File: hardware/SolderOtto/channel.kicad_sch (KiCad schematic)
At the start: 16 parts, among them J601 Conn_01x07

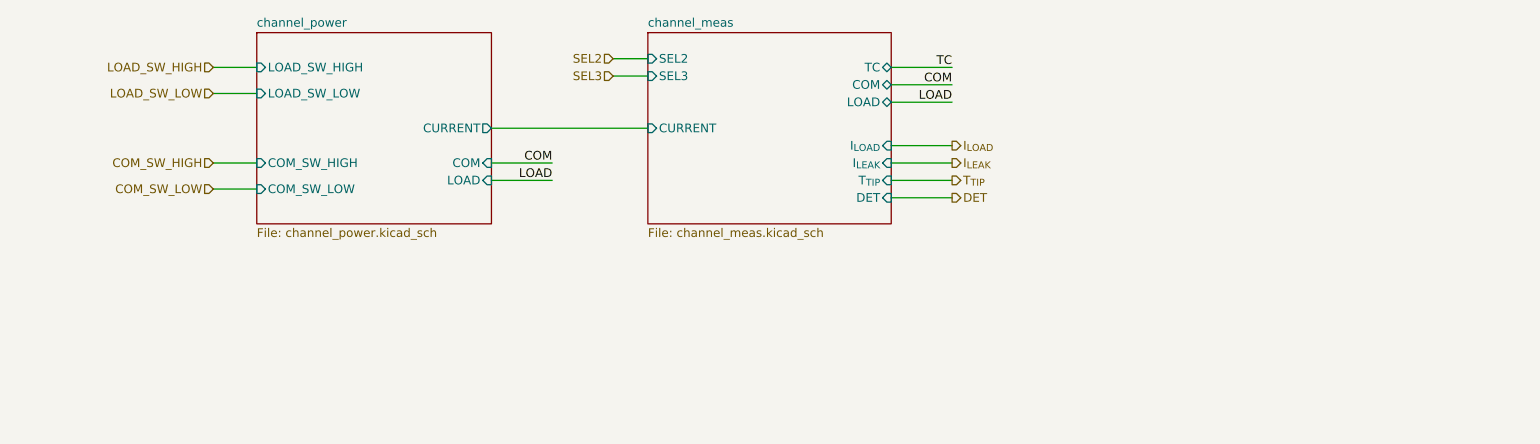
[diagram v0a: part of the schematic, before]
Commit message: save wip
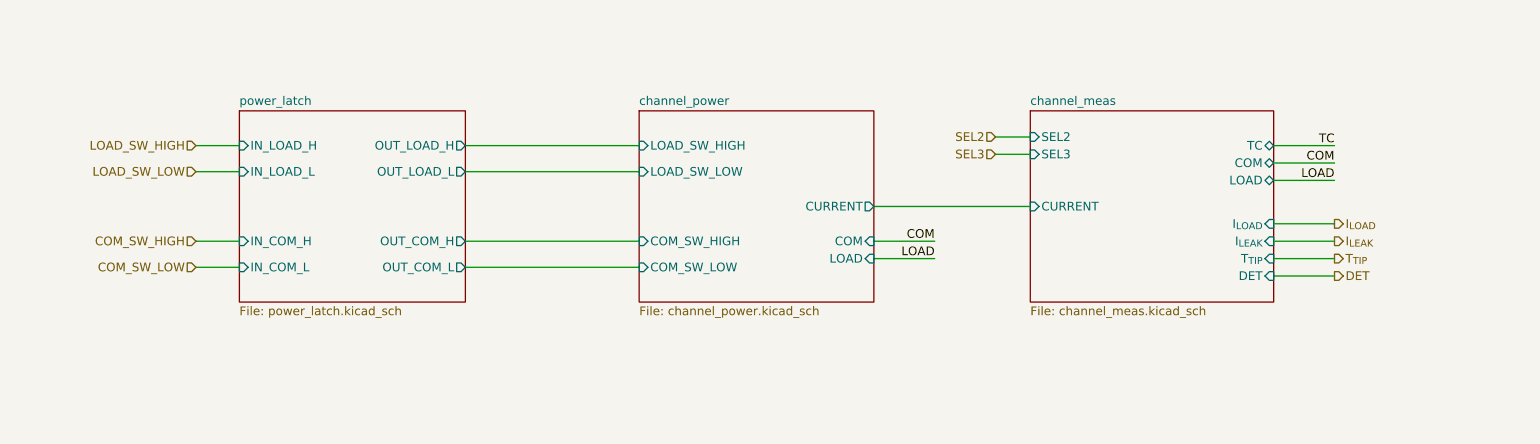
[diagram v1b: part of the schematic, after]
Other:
- added sheet power_latch (power_latch.kicad_sch)

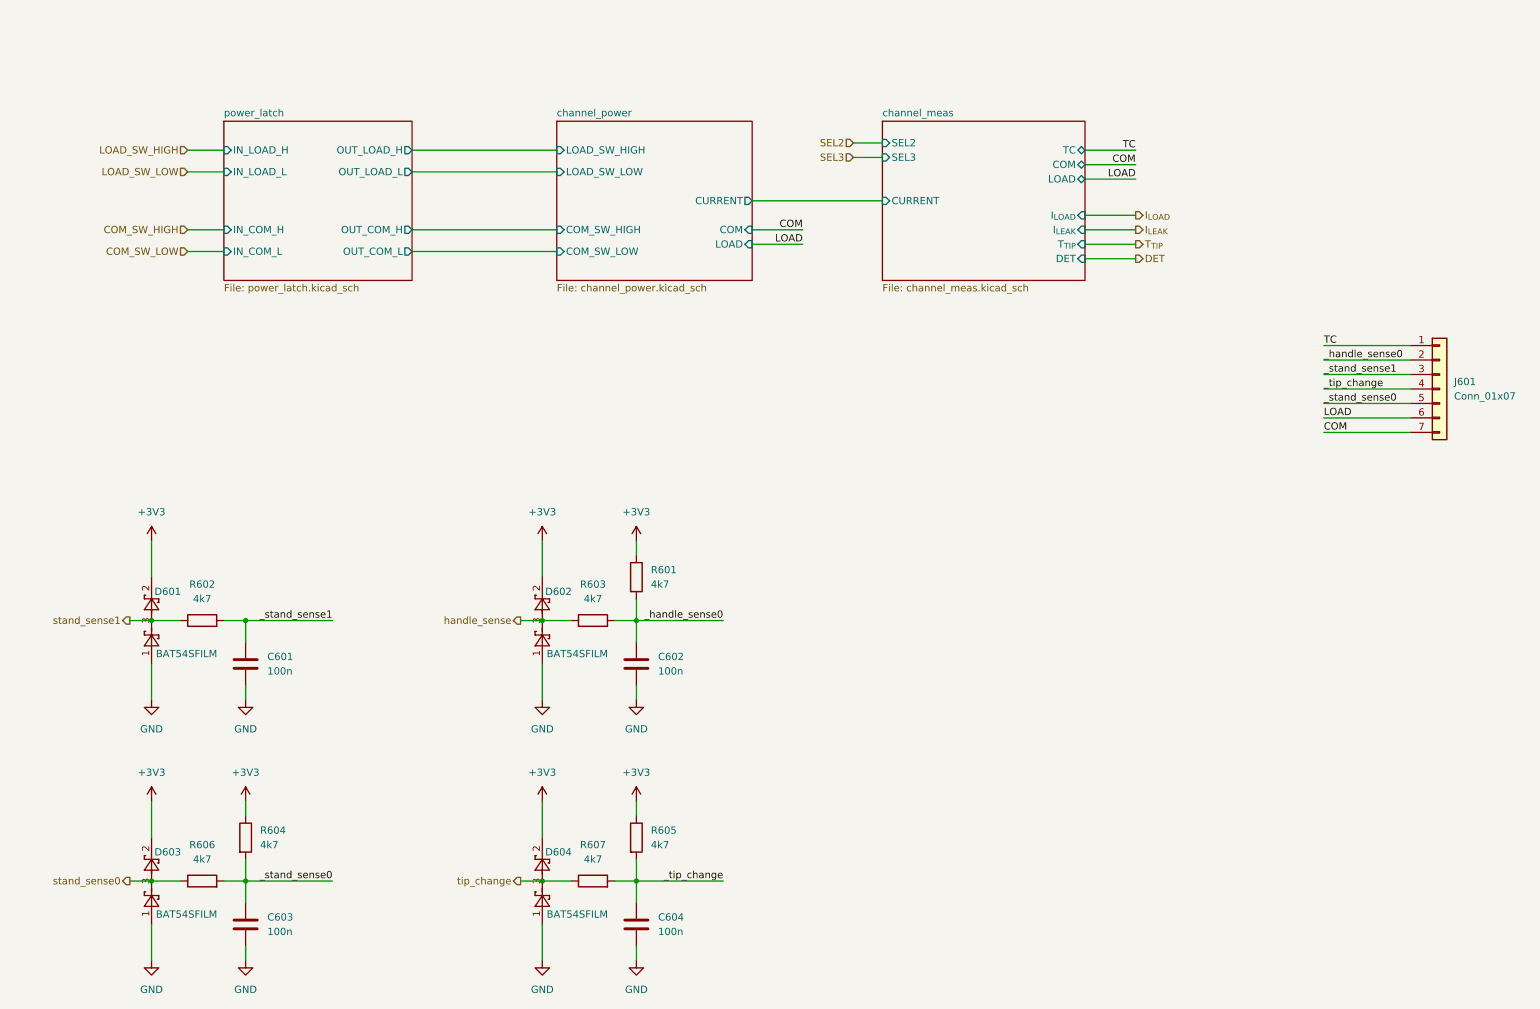
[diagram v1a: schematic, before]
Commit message: wip
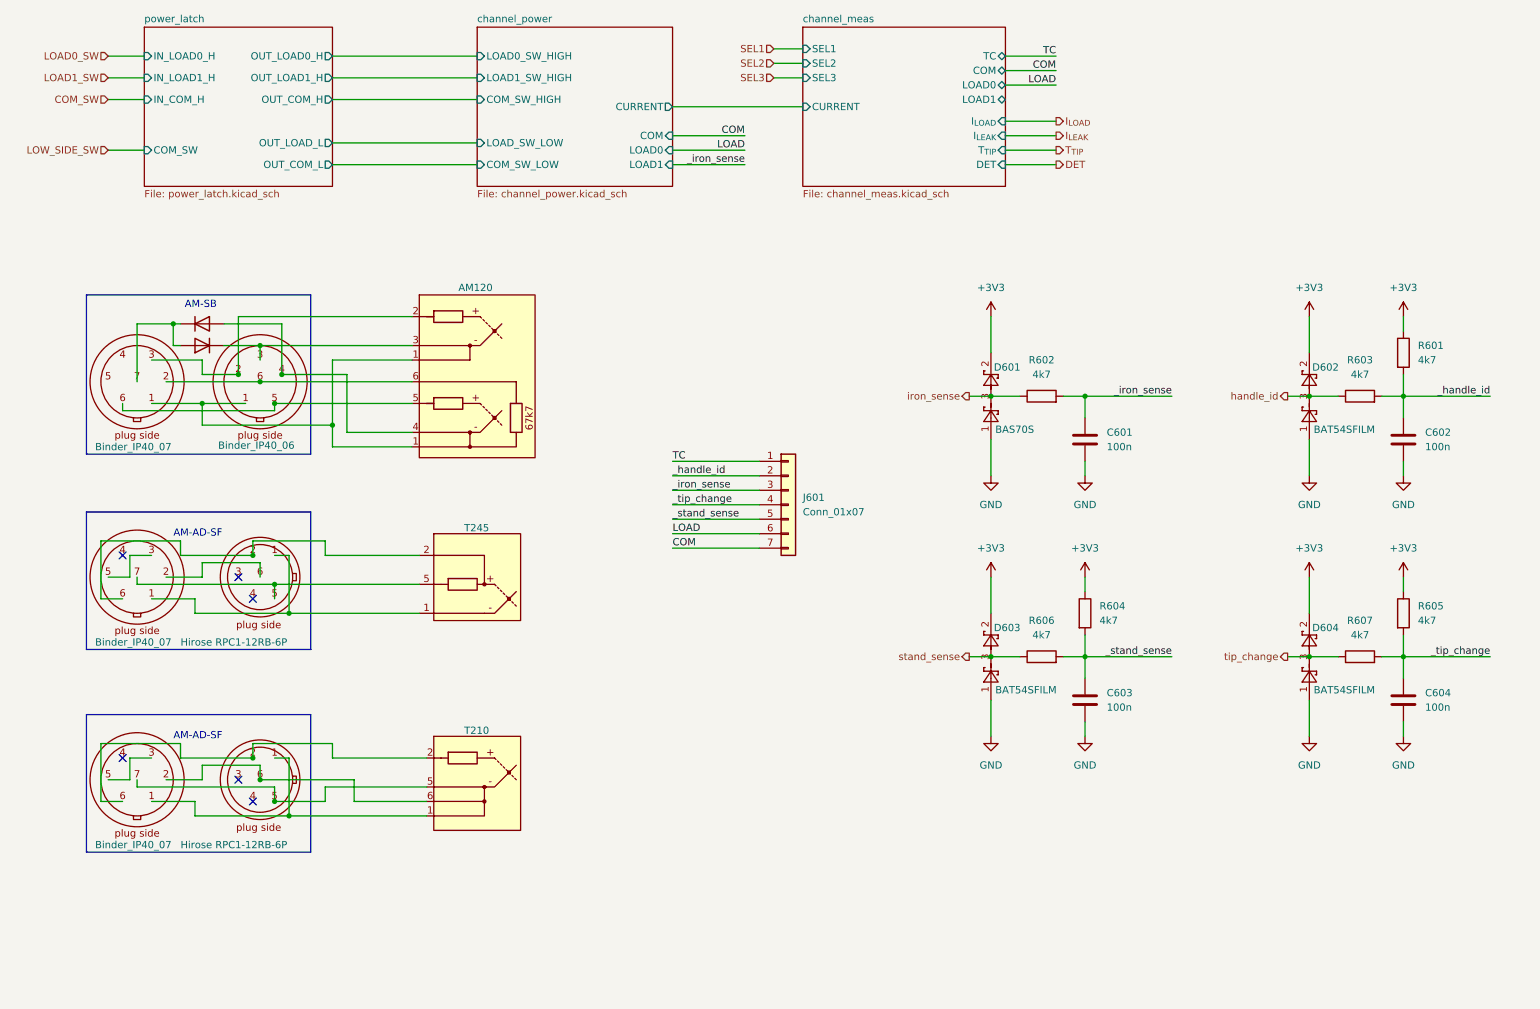
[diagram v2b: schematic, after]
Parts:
- added D605, D606: D, symbol Device:D
- added HEATER601: AM120, symbol mylib_connectors:JBC-AM120
- added HEATER602: T245, symbol mylib_connectors:JBC-T245
- added HEATER603: T210, symbol mylib_connectors:JBC-T210
- added X601, X603, X605: Binder_IP40_07, symbol mylib_connectors:Binder_IP40_07
- added X602: Binder_IP40_06, symbol mylib_connectors:Binder_IP40_06
- added X604, X606: Hirose RPC1-12RB-6P, symbol mylib_connectors:Hirose RPC1-12RB-6P
- D601: value BAT54SFILM -> BAS70S; Mouser 511-BAT54SFILM -> 3757-BAS70S_R1_00001CT-ND
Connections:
- net _handle_sense0 renamed _handle_id
- net _stand_sense0 renamed _stand_sense
- net _stand_sense1 renamed _iron_sense
- net handle_sense renamed handle_id
- net stand_sense0 renamed stand_sense
- net stand_sense1 renamed iron_sense
- new net: HEATER603.1, X605.1, X606.1
- new net: HEATER603.2, X605.6, X606.2
- new net: HEATER603.5, X605.7, X606.5
- new net: HEATER603.6, X605.2, X606.6
- new net: HEATER602.1, X603.1, X604.1
- new net: HEATER602.2, X603.6, X604.2
- new net: HEATER602.5, X603.7, X604.5
- new net: X603.2, X604.6
- new net: D605.1 (K), D606.2 (A), X601.7
- new net: D605.2 (A), HEATER601.4, X602.4
- new net: X605.3, X605.5
- new net: D606.1 (K), HEATER601.3, X602.3
- new net: HEATER601.1, X601.1, X602.1
- new net: HEATER601.2, X601.3, X602.2
- new net: HEATER601.5, X601.6, X602.5
- new net: HEATER601.6, X601.2, X602.6
- new net: X603.3, X603.5
- no-connect marks 0 -> 6
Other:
- sheet channel_meas ports: added LOAD0, LOAD1, SEL1; removed LOAD
- sheet channel_power ports: added LOAD0, LOAD0_SW_HIGH, LOAD1, LOAD1_SW_HIGH; removed LOAD, LOAD_SW_HIGH
- sheet power_latch ports: added COM_SW, IN_LOAD0_H, IN_LOAD1_H, OUT_LOAD0_H, OUT_LOAD1_H; removed IN_COM_L, IN_LOAD_H, IN_LOAD_L, OUT_LOAD_H
- note added: "AM-AD-SF"
- note added: "AM-SB"
- moved on the sheet: C601, C602, C603, C604, D601, D602, D603, D604, J601, R601, R602, R603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

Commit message: save wip
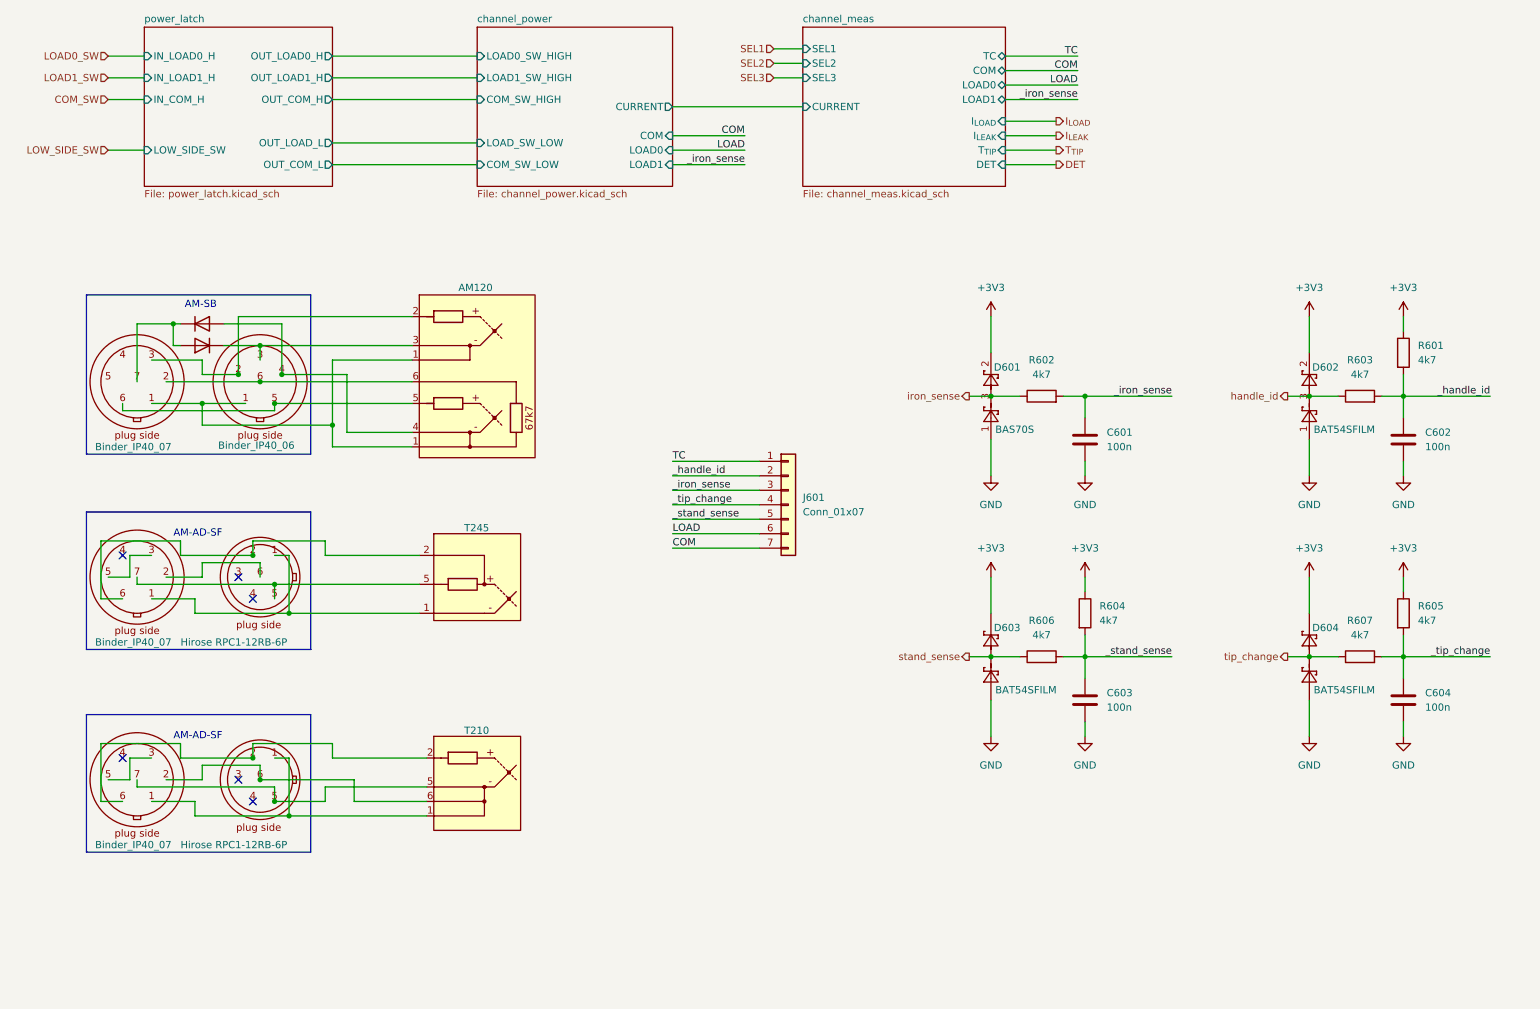
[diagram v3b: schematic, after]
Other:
- sheet power_latch ports: added LOW_SIDE_SW; removed COM_SW
